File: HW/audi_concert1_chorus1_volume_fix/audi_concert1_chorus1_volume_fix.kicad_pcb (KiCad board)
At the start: 2 copper layers, 33 x 27.2 mm, 44 parts, among them CON1 I2C_to_TDA, CON2 USB, CON3 SPI_TO_PANEL, CON4 JLINK, U1 68HC05_PLCC, U2 AP1117-33, U3 STM32F103C8Tx, U4 MAX809, Y1 32.768kHz, Y2 8MHz

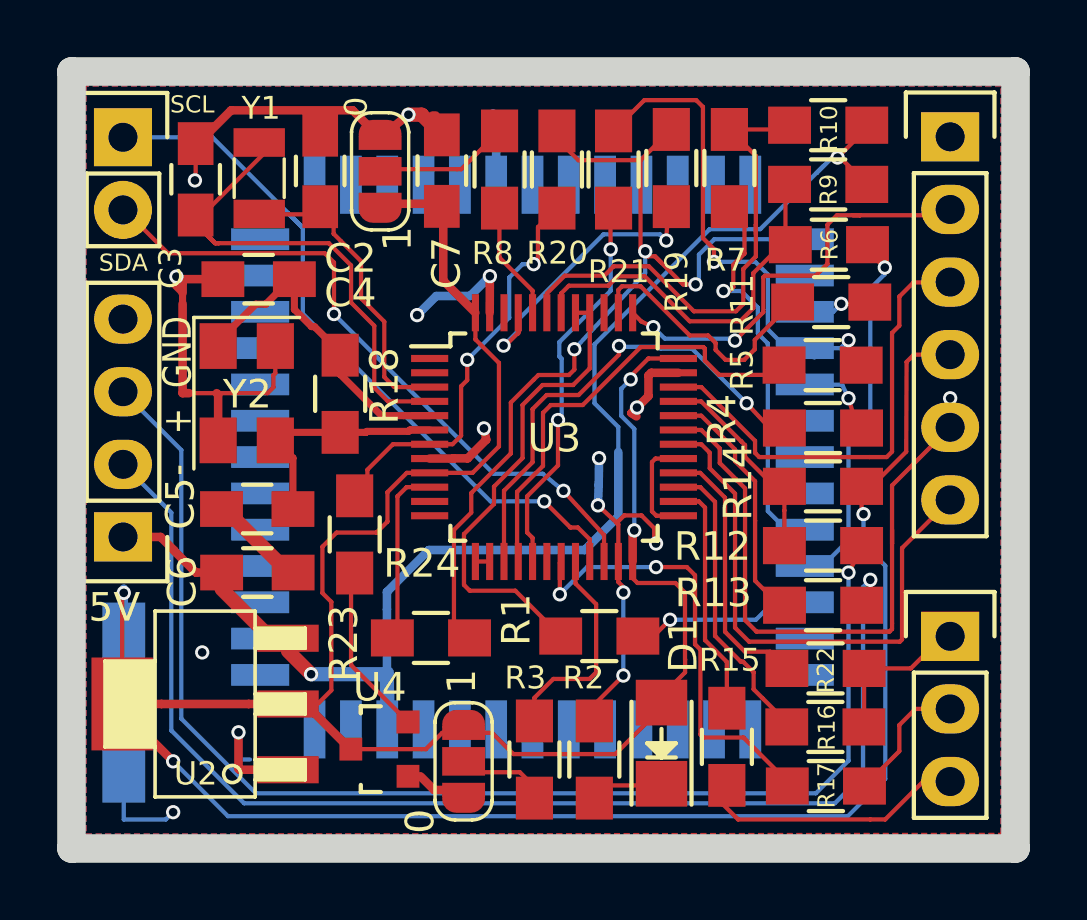
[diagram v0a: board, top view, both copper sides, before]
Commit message: kicad6
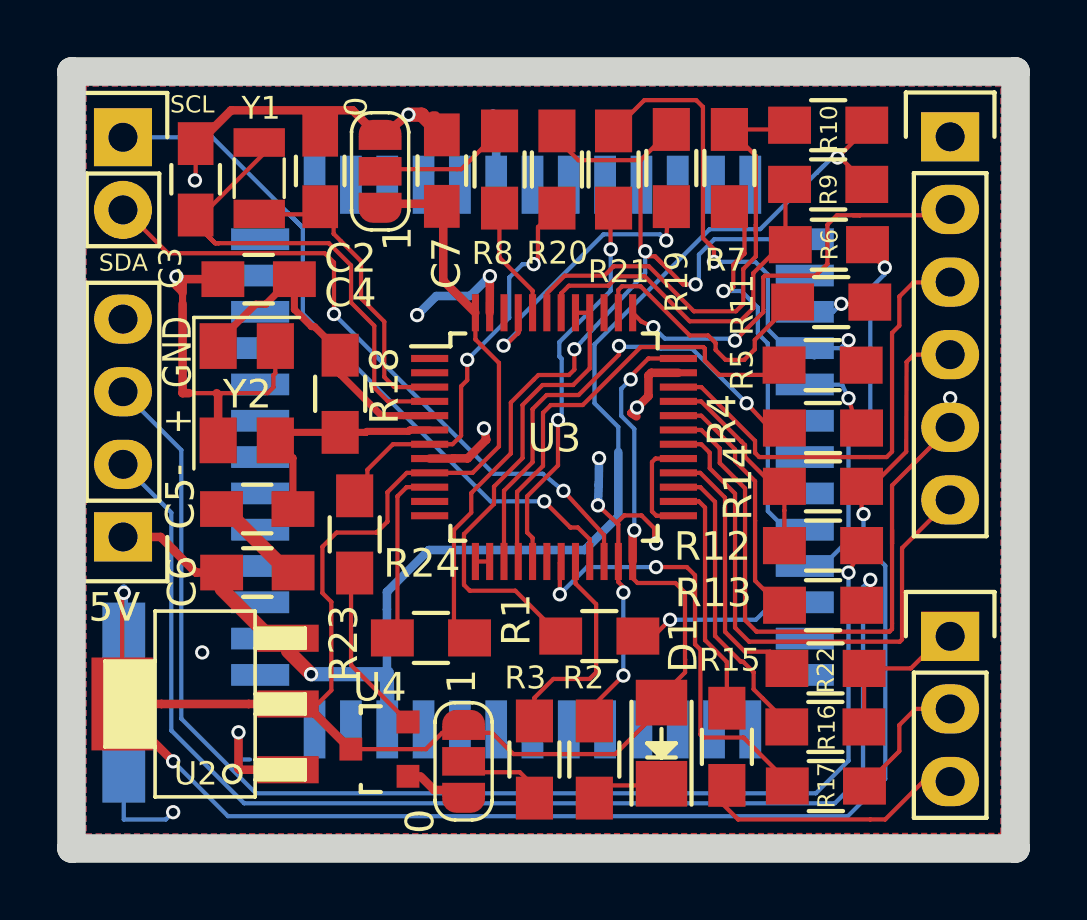
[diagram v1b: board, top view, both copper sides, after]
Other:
- net class 3v3 removed
- net class 5V removed
- net class Default removed
- net class GND removed
